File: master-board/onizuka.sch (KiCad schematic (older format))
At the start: 30 parts, among them IC1 FT232RQ, IC2 ADCMP371, P1 USB_OTG, P2 FTDI, Q1 Q_PMOS_GSD, SW1 SWITCH_INV, U1 MIC5353-3.3YMT

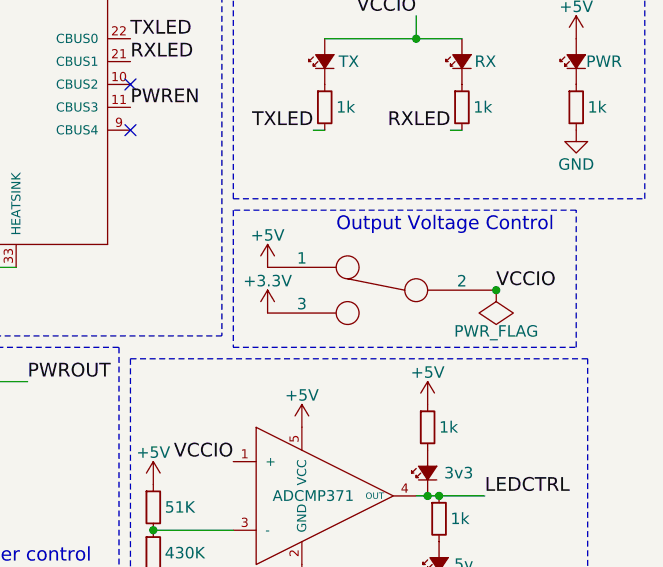
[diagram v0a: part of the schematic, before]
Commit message: Updated switch
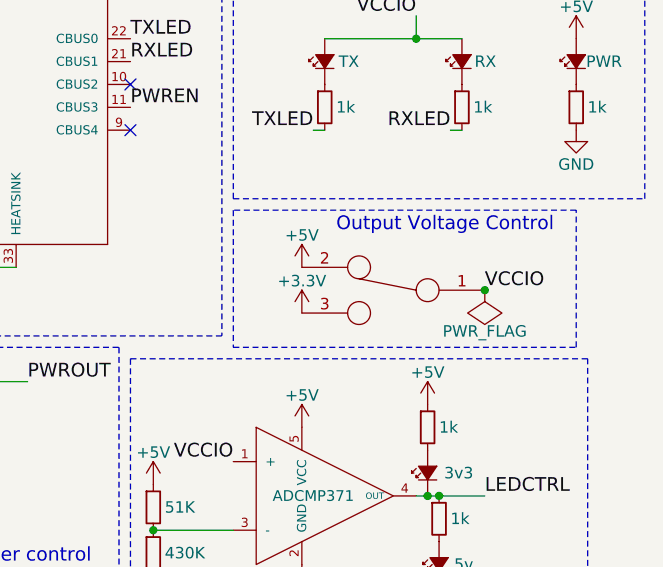
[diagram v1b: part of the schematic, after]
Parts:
- removed SW1: SWITCH_INV, Buttons_Switches_ThroughHole:SW_Micro_SPST, symbol SWITCH_INV
- added SW1: SPDT, Wurth:450301014042, symbol SPDT
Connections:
- net +3V3: now also SW1.3
- net +5V: now also SW1.2
- net VCCIO: now also SW1.1
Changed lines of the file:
@@
 LIBS:contrib
 LIBS:valves
-LIBS:ftdi
 LIBS:ad
 LIBS:micrel
-LIBS:power-ext
+LIBS:ftdi
+LIBS:Switches
 LIBS:onizuka-cache
 EELAYER 25 0
@@
 $EndComp
 $Comp
-L SWITCH_INV SW1
-U 1 1 573F1E28
-P 5500 2850
-F 0 "SW1" H 5300 3000 50  0001 C CNN
-F 1 "SWITCH_INV" H 5350 2700 50  0001 C CNN
-F 2 "Buttons_Switches_ThroughHole:SW_Micro_SPST" H 5500 2850 50  0001 C CNN
-F 3 "" H 5500 2850 50  0000 C CNN
-	1    5500 2850
-	-1   0    0    -1
-$EndComp
-$Comp
 L +5V #PWR010
 U 1 1 573F1E7D
-P 5000 2750
-F 0 "#PWR010" H 5000 2600 50  0001 C CNN
-F 1 "+5V" H 5000 2890 50  0000 C CNN
-F 2 "" H 5000 2750 50  0000 C CNN
-F 3 "" H 5000 2750 50  0000 C CNN
-	1    5000 2750
+P 5150 2750
+F 0 "#PWR010" H 5150 2600 50  0001 C CNN
+F 1 "+5V" H 5150 2890 50  0000 C CNN
+F 2 "" H 5150 2750 50  0000 C CNN
+F 3 "" H 5150 2750 50  0000 C CNN
+	1    5150 2750
 	-1   0    0    -1
 $EndComp
@@
 L +3.3V #PWR011
 U 1 1 573F1E91
-P 5000 2950
-F 0 "#PWR011" H 5000 2800 50  0001 C CNN
-F 1 "+3.3V" H 5000 3090 50  0000 C CNN
-F 2 "" H 5000 2950 50  0000 C CNN
-F 3 "" H 5000 2950 50  0000 C CNN
-	1    5000 2950
+P 5150 2950
+F 0 "#PWR011" H 5150 2800 50  0001 C CNN
+F 1 "+3.3V" H 5150 3090 50  0000 C CNN
+F 2 "" H 5150 2950 50  0000 C CNN
+F 3 "" H 5150 2950 50  0000 C CNN
+	1    5150 2950
 	-1   0    0    -1
 $EndComp
-Text Label 6000 2850 0    60   ~ 0
+Text Label 5950 2850 0    60   ~ 0
 VCCIO
 Text Label 2900 3250 2    60   ~ 0
@@
 L PWR_FLAG #FLG013
 U 1 1 573F27A3
-P 6000 2850
-F 0 "#FLG013" H 6000 2945 50  0001 C CNN
-F 1 "PWR_FLAG" H 6000 3030 50  0000 C CNN
-F 2 "" H 6000 2850 50  0000 C CNN
-F 3 "" H 6000 2850 50  0000 C CNN
-	1    6000 2850
+P 5950 2850
+F 0 "#FLG013" H 5950 2945 50  0001 C CNN
+F 1 "PWR_FLAG" H 5950 3030 50  0000 C CNN
+F 2 "" H 5950 2850 50  0000 C CNN
+F 3 "" H 5950 2850 50  0000 C CNN
+	1    5950 2850
 	-1   0    0    1
 $EndComp
@@
 	1    0    0    -1
 $EndComp
-Connection ~ 6000 2850
+Connection ~ 5950 2850
 $Comp
 L FT232RQ IC1
@@
 	1    0    0    -1
 $EndComp
+$Comp
+L SPDT SW1
+U 1 1 574EF3CB
+P 5550 2850
+F 0 "SW1" H 5550 2500 60  0001 C CNN
+F 1 "SPDT" H 5550 3150 60  0001 C CNN
+F 2 "Wurth:450301014042" H 5600 2850 60  0001 C CNN
+F 3 "" H 5600 2850 60  0000 C CNN
+	1    5550 2850
+	1    0    0    -1
+$EndComp
